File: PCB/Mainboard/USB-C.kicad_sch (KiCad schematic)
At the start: 21 parts, among them J1 TYPE-C-31-M-12, Q1 AON7262E, Q2 AON7262E, U3 TPD4E05U06DQA

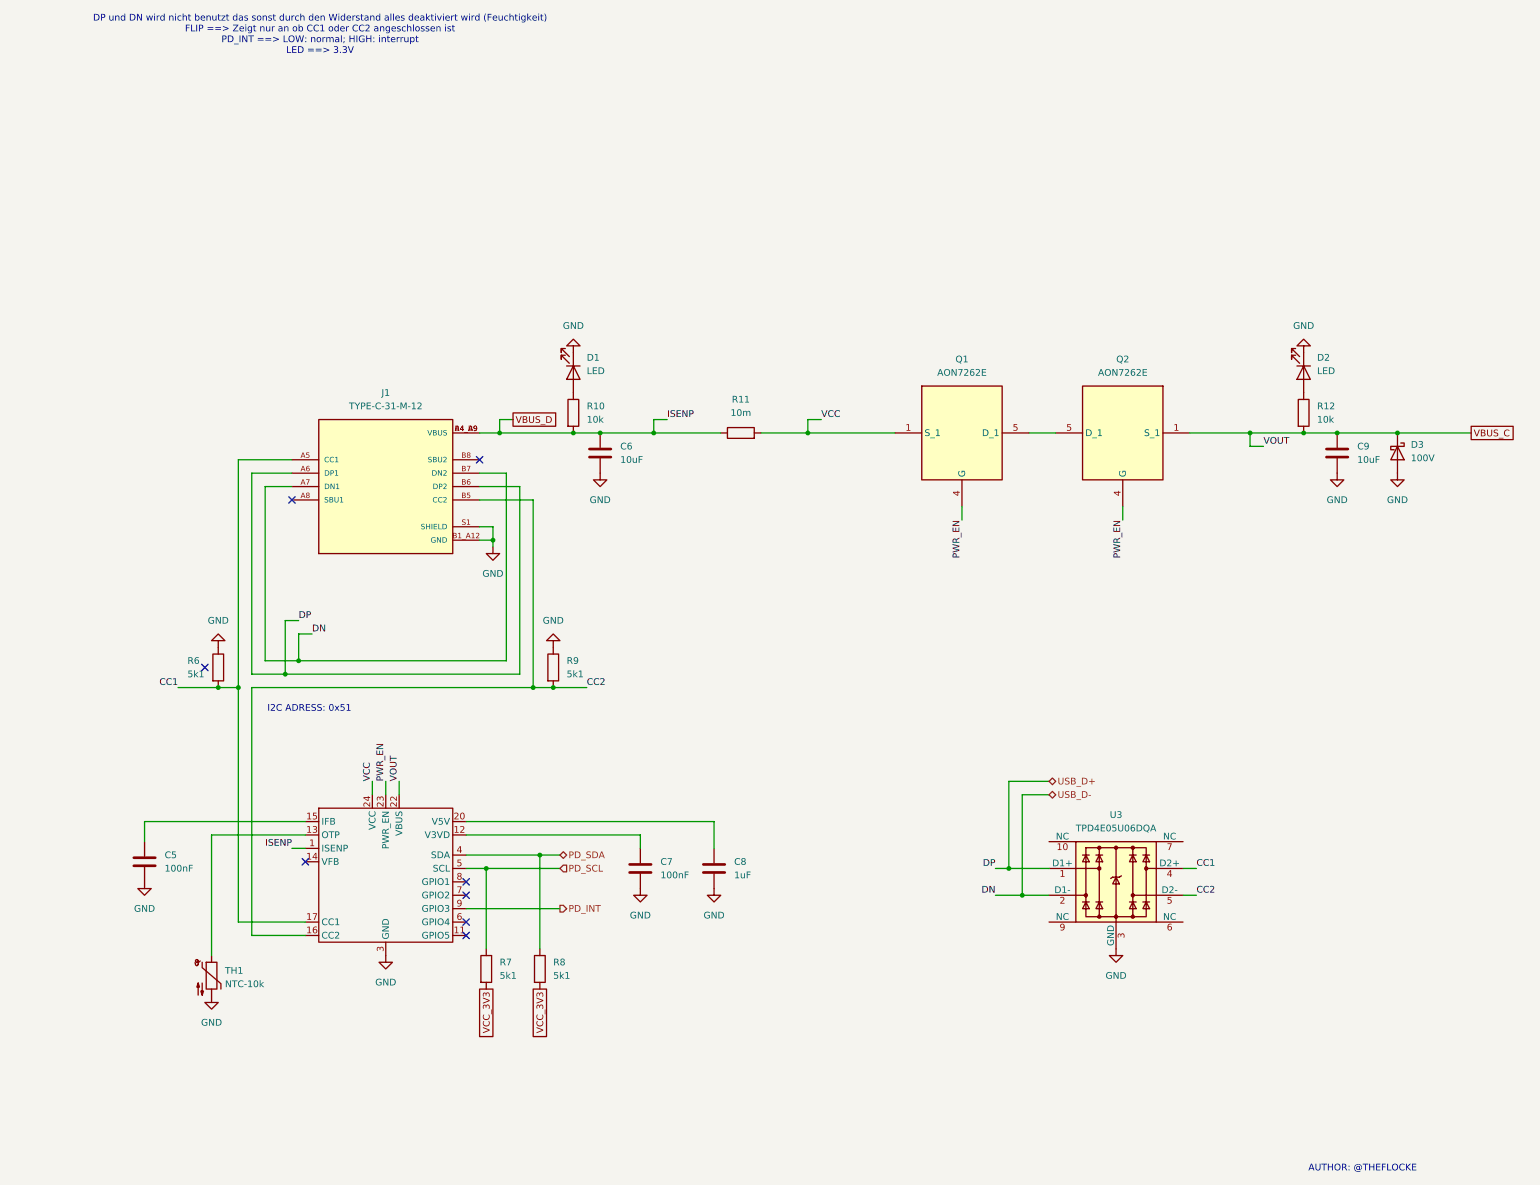
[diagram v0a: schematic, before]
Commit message: Fixed Grammar
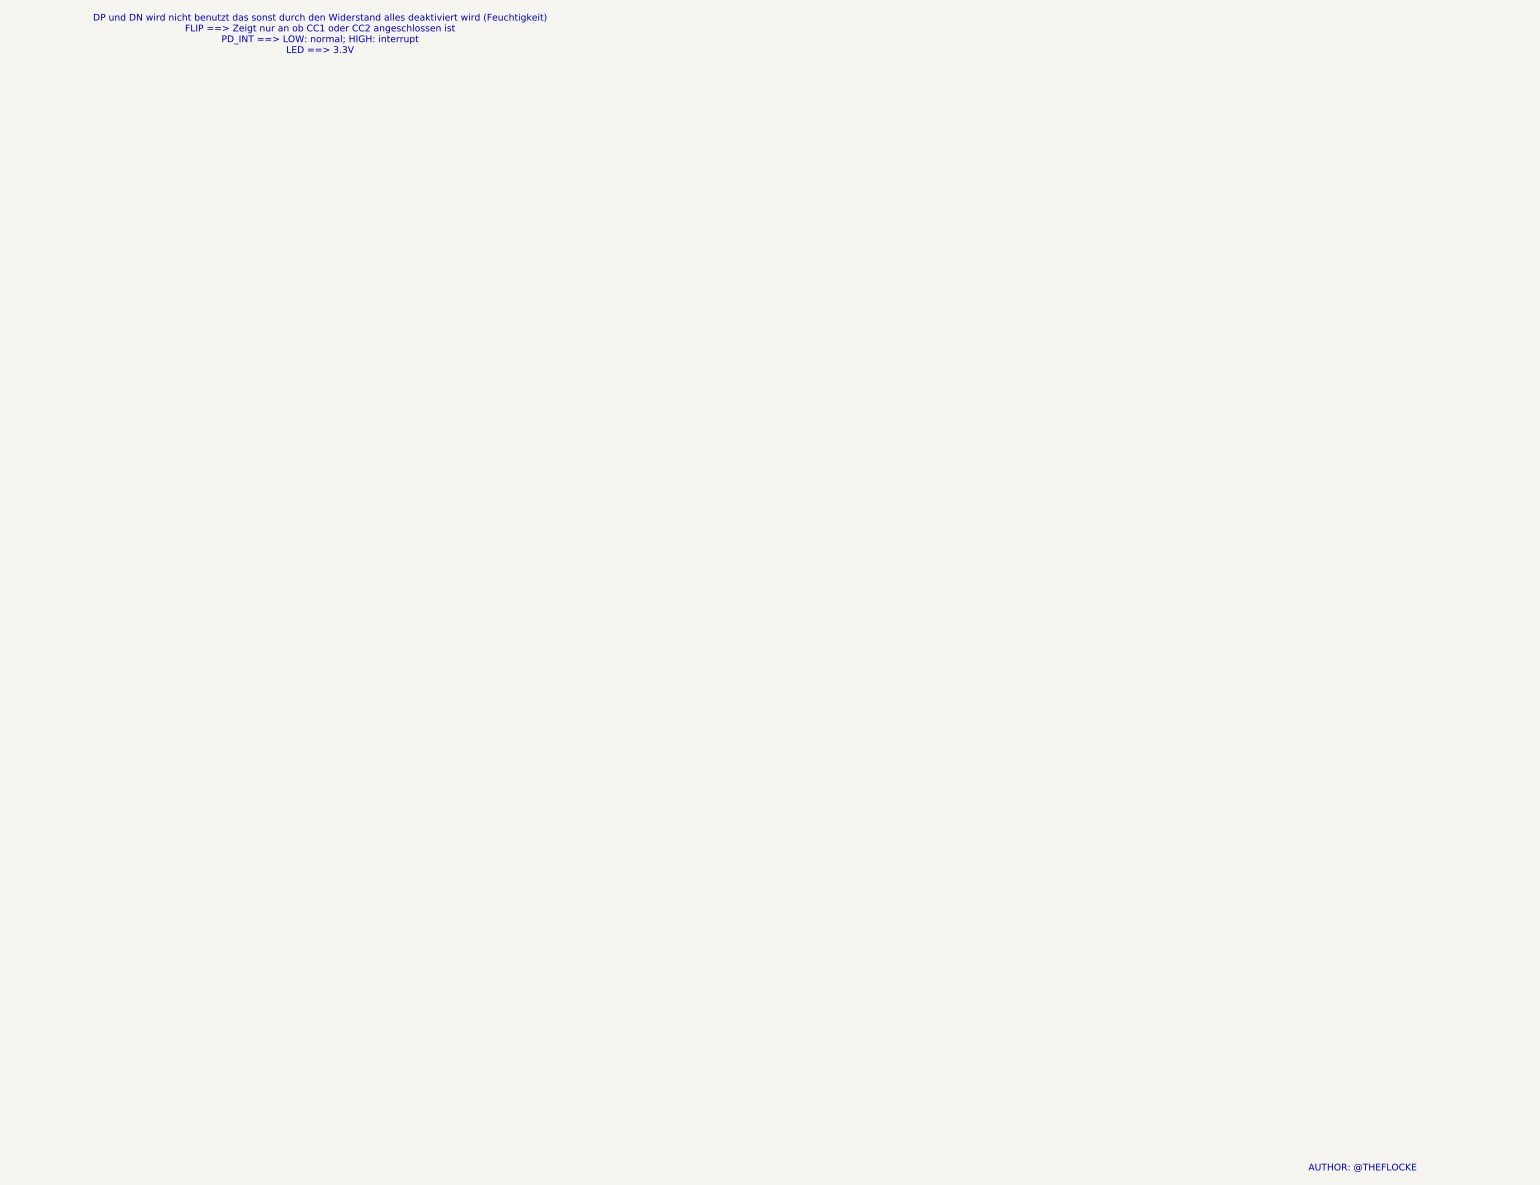
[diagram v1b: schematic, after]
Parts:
- removed C5, C7: 100nF, Capacitor_SMD:C_0805_2012Metric_Pad1.18x1.45mm_HandSolder, symbol Device:C
- removed C6, C9: 10uF, Capacitor_SMD:C_0805_2012Metric_Pad1.18x1.45mm_HandSolder, symbol Device:C
- removed C8: 1uF, Capacitor_SMD:C_0805_2012Metric_Pad1.18x1.45mm_HandSolder, symbol Device:C
- removed D1, D2: LED, Diode_SMD:D_0805_2012Metric_Pad1.15x1.40mm_HandSolder, symbol Device:LED
- removed D3: 100V, Diode_SMD:D_SMA, symbol Device:D_Schottky
- removed J1: TYPE-C-31-M-12, Footprints:HRO_TYPE-C-31-M-12, symbol TYPE-C-31-M-12:TYPE-C-31-M-12
- removed Q1, Q2: AON7262E, AON7262E, symbol AON7262E:AON7262E
- removed R10, R12: 10k, Resistor_SMD:R_0805_2012Metric_Pad1.20x1.40mm_HandSolder, symbol Device:R
- removed R11: 10m, Resistor_SMD:R_0805_2012Metric_Pad1.20x1.40mm_HandSolder, symbol Device:R
- removed R6, R7, R8, R9: 5k1, Resistor_SMD:R_0805_2012Metric_Pad1.20x1.40mm_HandSolder, symbol Device:R
- removed TH1: NTC-10k, Resistor_SMD:R_0805_2012Metric_Pad1.20x1.40mm_HandSolder, symbol Device:Thermistor_NTC
- removed U2: ~, custom:AP33772, symbol Custom:AP33772
- removed U3: TPD4E05U06DQA, Package_SON:USON-10_2.5x1.0mm_P0.5mm, symbol Power_Protection:TPD4E05U06DQA
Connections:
- no-connect marks 8 -> 0
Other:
- note removed: "I2C ADRESS: 0x51"

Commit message: upload images and deleted pcb new
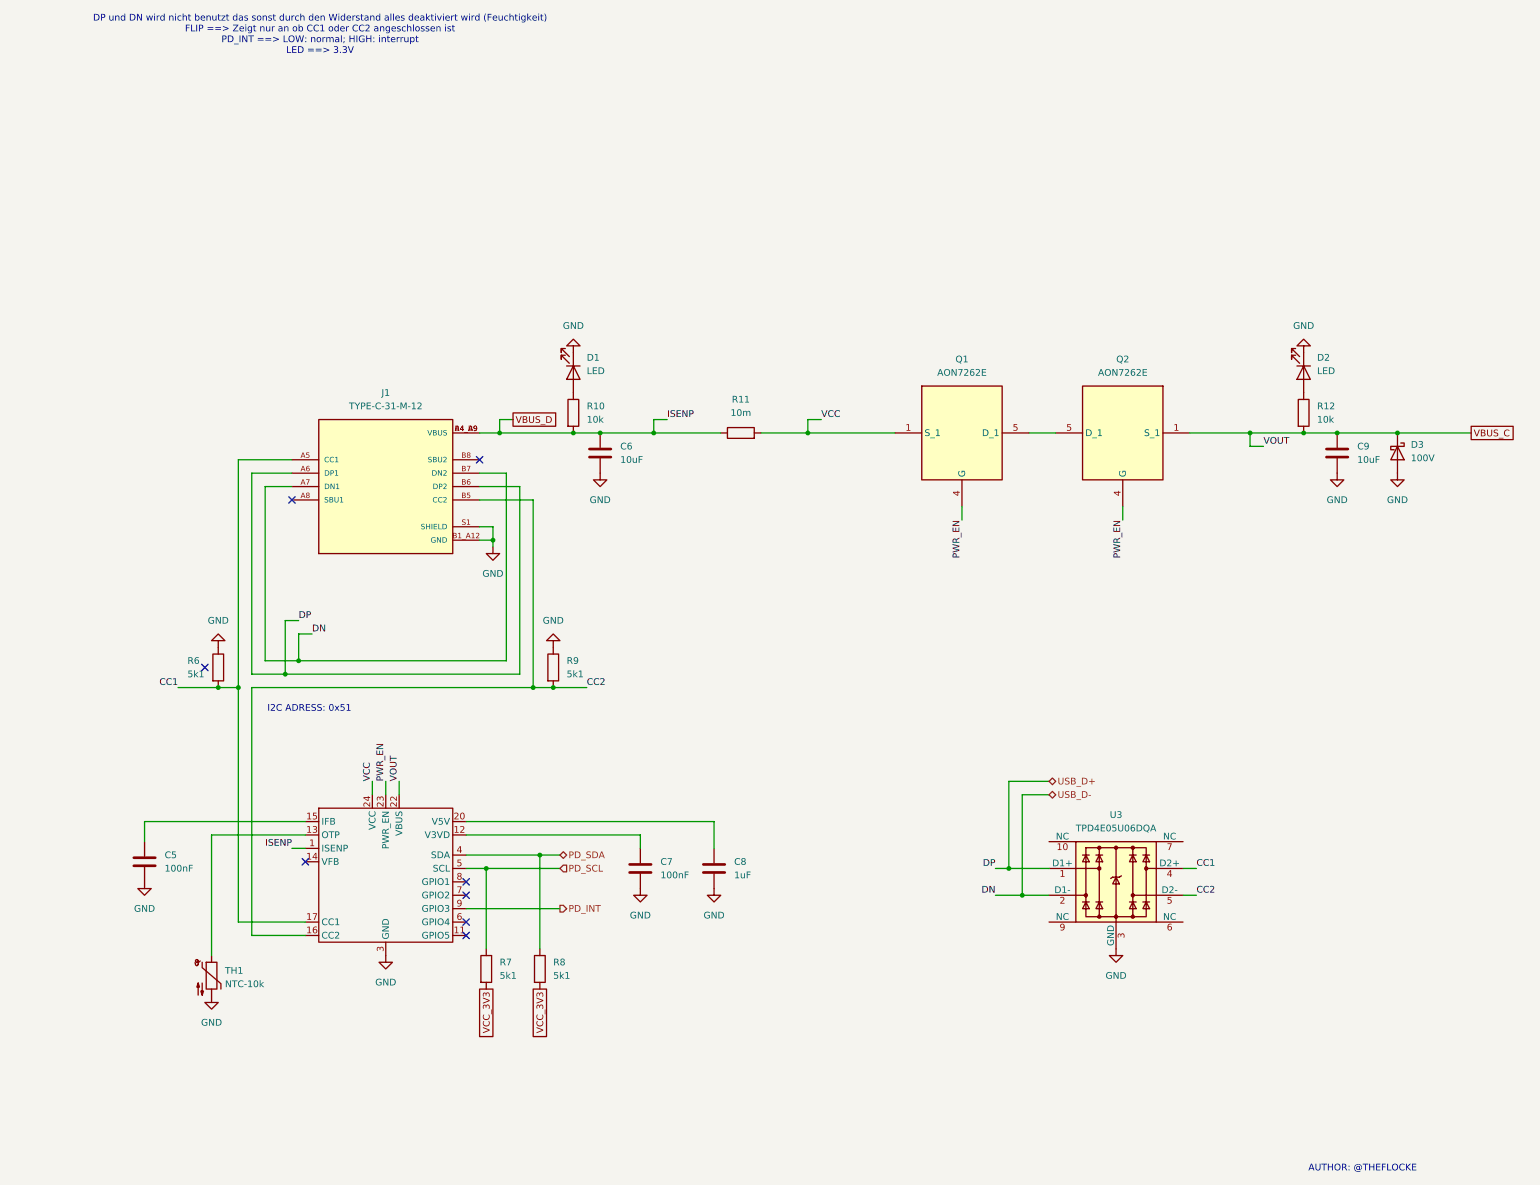
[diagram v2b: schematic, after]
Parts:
- added C5, C7: 100nF, Capacitor_SMD:C_0805_2012Metric_Pad1.18x1.45mm_HandSolder, symbol Device:C
- added C6, C9: 10uF, Capacitor_SMD:C_0805_2012Metric_Pad1.18x1.45mm_HandSolder, symbol Device:C
- added C8: 1uF, Capacitor_SMD:C_0805_2012Metric_Pad1.18x1.45mm_HandSolder, symbol Device:C
- added D1, D2: LED, Diode_SMD:D_0805_2012Metric_Pad1.15x1.40mm_HandSolder, symbol Device:LED
- added D3: 100V, Diode_SMD:D_SMA, symbol Device:D_Schottky
- added J1: TYPE-C-31-M-12, Footprints:HRO_TYPE-C-31-M-12, symbol TYPE-C-31-M-12:TYPE-C-31-M-12
- added Q1, Q2: AON7262E, AON7262E, symbol AON7262E:AON7262E
- added R10, R12: 10k, Resistor_SMD:R_0805_2012Metric_Pad1.20x1.40mm_HandSolder, symbol Device:R
- added R11: 10m, Resistor_SMD:R_0805_2012Metric_Pad1.20x1.40mm_HandSolder, symbol Device:R
- added R6, R7, R8, R9: 5k1, Resistor_SMD:R_0805_2012Metric_Pad1.20x1.40mm_HandSolder, symbol Device:R
- added TH1: NTC-10k, Resistor_SMD:R_0805_2012Metric_Pad1.20x1.40mm_HandSolder, symbol Device:Thermistor_NTC
- added U2: ~, custom:AP33772, symbol Custom:AP33772
- added U3: TPD4E05U06DQA, Package_SON:USON-10_2.5x1.0mm_P0.5mm, symbol Power_Protection:TPD4E05U06DQA
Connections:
- new net: D1.2 (A), R10.1
- new net: D2.2 (A), R12.1
- new net: Q1.10 (D_6), Q1.11 (D_7), Q1.5 (D_1), Q1.6 (D_2), Q1.7 (D_3), Q1.8 (D_4), Q1.9 (D_5), Q2.10 (D_6), Q2.11 (D_7), Q2.5 (D_1), Q2.6 (D_2), Q2.7 (D_3), Q2.8 (D_4), Q2.9 (D_5)
- new net: C5.1, U2.15 (IFB)
- new net: U2.10 (NC), U2.18 (NC), U2.19 (NC), U2.2 (NC), U2.21 (NC)
- new net: C7.1, U2.12 (V3VD)
- new net: TH1.1, U2.13 (OTP)
- new net: C8.1, U2.20 (V5V)
- new net CC1: J1.A5 (CC1), R6.2, U2.17 (CC1), U3.4 (D2+)
- new net CC2: J1.B5 (CC2), R9.2, U2.16 (CC2), U3.5 (D2-)
- new net GND: C5.2, C6.2, C7.2, C8.2, C9.2, D1.1 (K), D2.1 (K), D3.2 (A), J1.A1_B12 (GND), J1.B1_A12 (GND), J1.S1 (SHIELD), J1.S2 (SHIELD), J1.S3 (SHIELD), J1.S4 (SHIELD), R6.1, R9.1, TH1.2, U2.3 (GND), U3.3 (GND), U3.8 (GND)
- new net PD_INT: U2.9 (GPIO3)
- new net PD_SCL: R7.1, U2.5 (SCL)
- new net PD_SDA: R8.1, U2.4 (SDA)
- new net PWR_EN: Q1.4 (G), Q2.4 (G), U2.23 (PWR_EN)
- new net USB_D+: J1.A6 (DP1), J1.B6 (DP2), U3.1 (D1+)
- new net USB_D-: J1.A7 (DN1), J1.B7 (DN2), U3.2 (D1-)
- new net VBUS_C: C9.1, D3.1 (K), Q2.1 (S_1), Q2.2 (S_2), Q2.3 (S_3), R12.2, U2.22 (VBUS)
- new net VBUS_D: C6.1, J1.A4_B9 (VBUS), J1.B4_A9 (VBUS), R10.2, R11.1, U2.1 (ISENP)
- new net VCC: Q1.1 (S_1), Q1.2 (S_2), Q1.3 (S_3), R11.2, U2.24 (VCC)
- new net VCC_3V3: R7.2, R8.2
- no-connect marks 0 -> 8
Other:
- note added: "I2C ADRESS: 0x51"
